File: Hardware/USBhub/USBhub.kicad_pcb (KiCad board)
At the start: 2 copper layers, 45 x 4 mm, 23 parts, among them J3 USB_A, J4 USB_A, U1 NUP4202, U2 USB2512B-I/M2, U3 NUP4202, U4 NUP4202

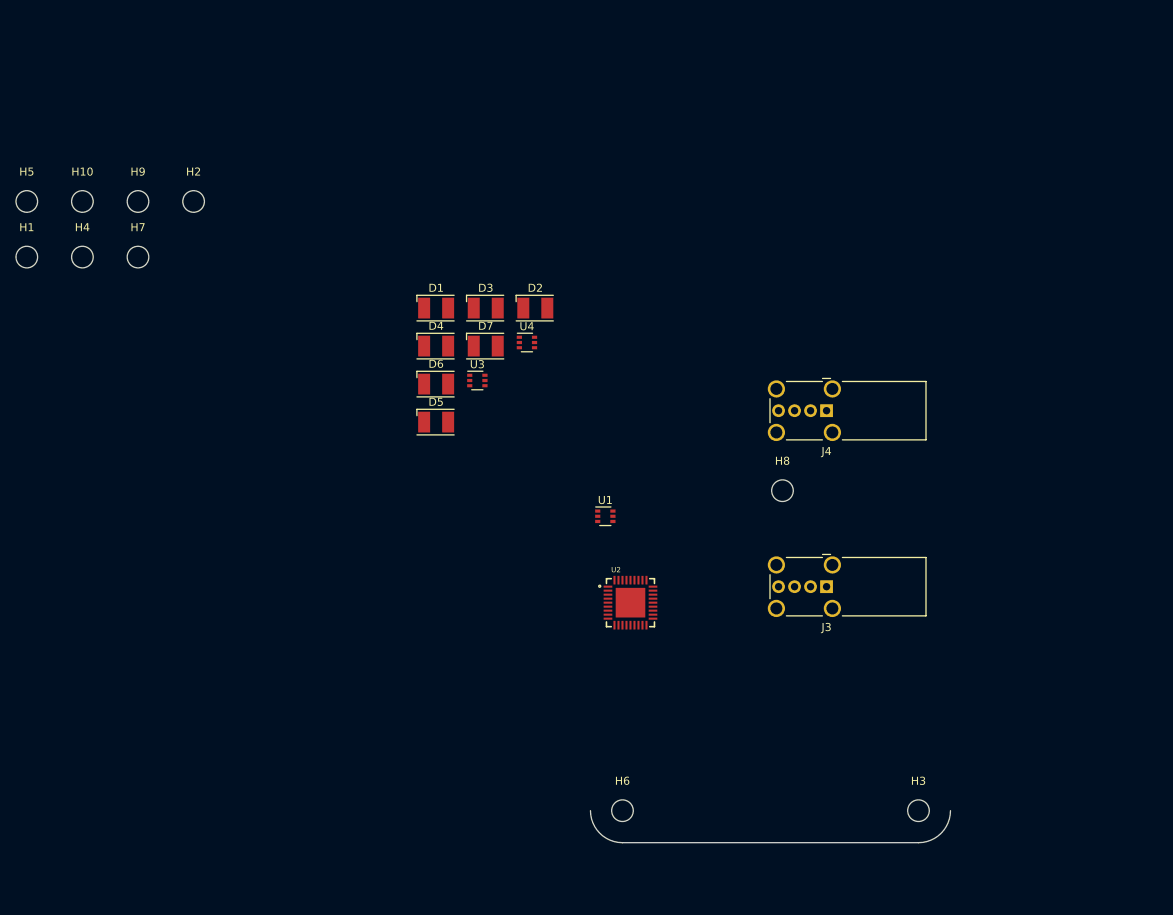
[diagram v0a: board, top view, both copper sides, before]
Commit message: small updates
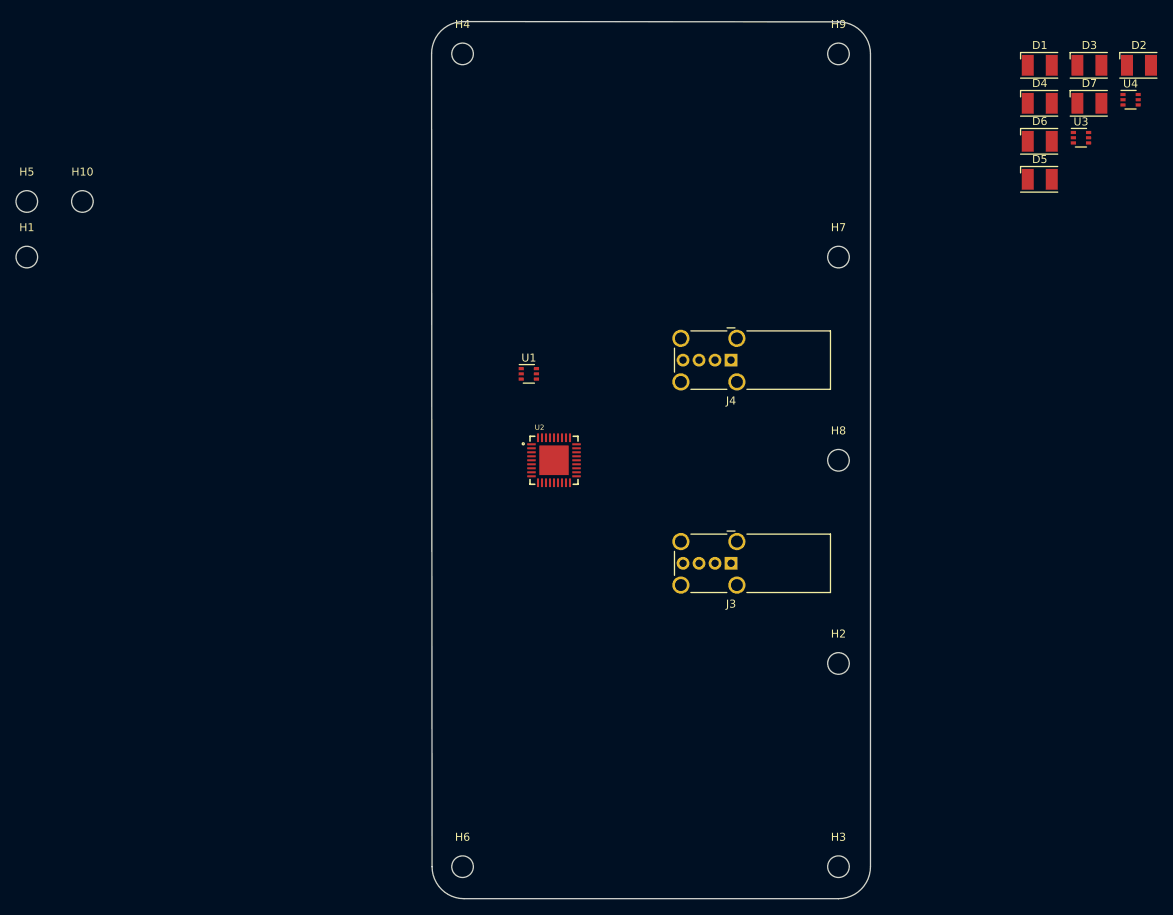
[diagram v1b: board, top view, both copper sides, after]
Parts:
- moved H2 99.2 mm to (127.0, 101.6)
- moved H9 89.5 mm to (127.0, 25.4)
- moved H7 87.6 mm to (127.0, 50.8)
- moved D3 81.3 mm to (158.4, 26.8)
- moved D7 81.3 mm to (158.4, 31.6)
- moved D1 81.3 mm to (152.2, 26.8)
- moved D2 81.3 mm to (164.6, 26.8)
- moved D4 81.3 mm to (152.2, 31.6)
- moved D5 81.3 mm to (152.2, 41.1)
- moved D6 81.3 mm to (152.2, 36.3)
- moved U3 81.3 mm to (157.3, 35.9)
- moved U4 81.3 mm to (163.5, 31.1)
- moved H4 53.9 mm to (80.0, 25.4)
- moved H6 21.2 mm to (80.0, 127.0)
- moved U2 20.2 mm to (91.4, 76.2)
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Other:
- board size 45 x 4 mm -> 54.9 x 109.6 mm
